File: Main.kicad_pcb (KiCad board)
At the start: 2 copper layers, 71.1 x 34.3 mm, 12 parts, among them P1 CONN_01X06, U3 BLE_NANO

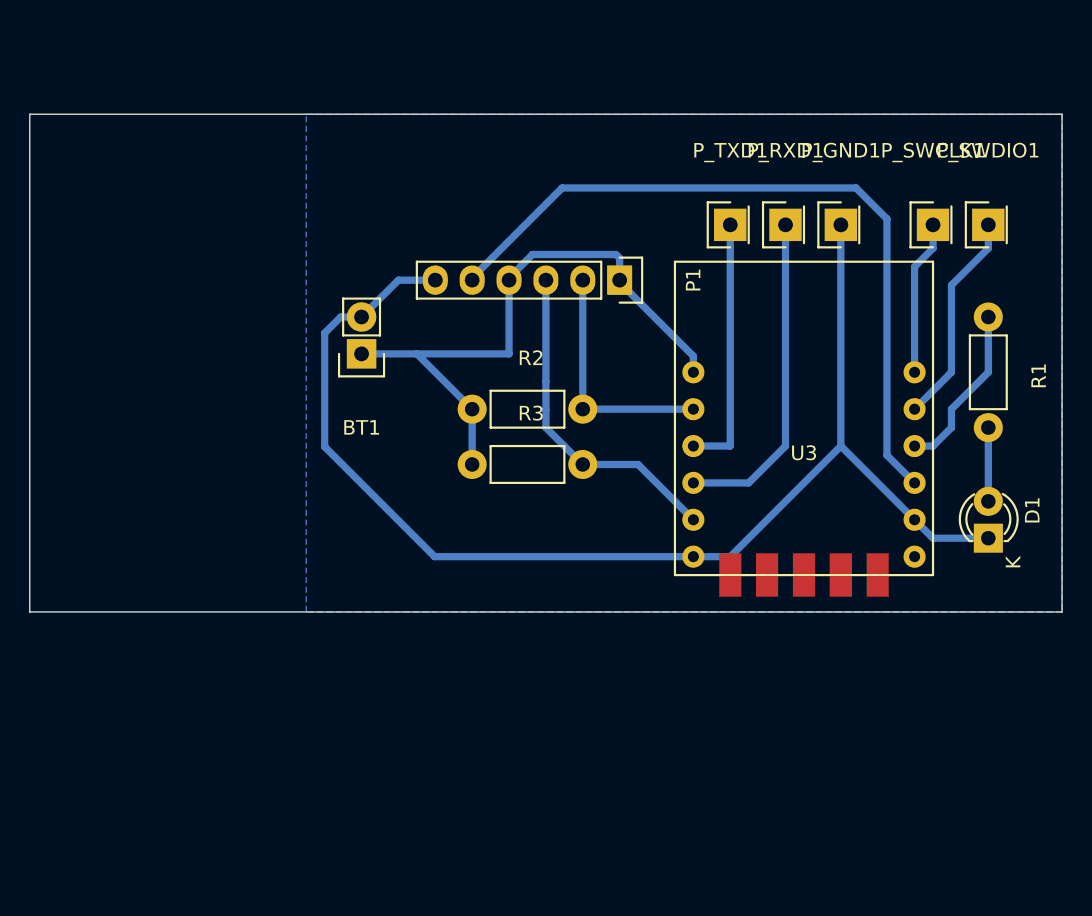
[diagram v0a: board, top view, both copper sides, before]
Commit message: update
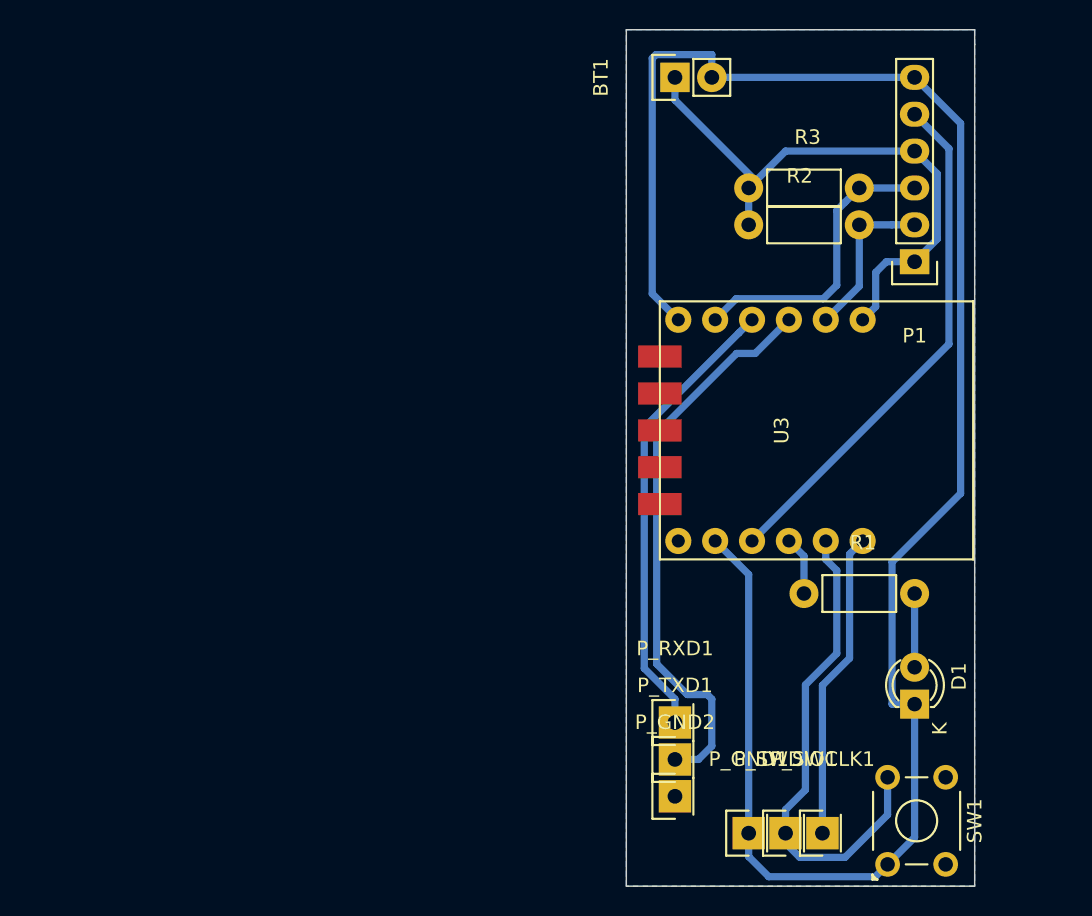
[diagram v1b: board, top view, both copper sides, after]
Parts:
- added P_GND2: CONN_01X01, Socket_Strips:Socket_Strip_Straight_1x01, F.Cu at (133.3, 130.8)
- added SW1: SW_RESET, Buttons_Switches_ThroughHole:SW_TH_Tactile_Omron_B3F-10xx, F.Cu at (148.0, 135.5)
- R1: value 10 -> 4.7k
- moved P_SWDIO1 44.2 mm to (141.0, 133.3)
- moved P_SWCLK1 42.6 mm to (143.5, 133.3)
- moved P_GND1 42.4 mm to (138.4, 133.3)
- moved P_TXD1 37.0 mm to (133.3, 128.3)
- moved P_RXD1 35.1 mm to (133.3, 125.7)
- moved BT1 28.8 mm to (133.3, 81.3), turned to 90 degrees
- moved R3 26.9 mm to (138.4, 88.9)
- moved R2 22.9 mm to (138.4, 91.4)
- moved R1 22.9 mm to (142.2, 116.8), turned to 0 degrees
- moved P1 20.4 mm to (149.9, 94.0), turned to 180 degrees
- moved D1 12.5 mm to (149.9, 124.5)
- moved U3 1.50 mm to (141.2, 105.6), turned to 270 degrees
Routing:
- net GND: track 86.8 -> 131.5 mm
- net /Main/TXD: track 17.8 -> 39.2 mm
- net /Main/SWDIO: track 14.8 -> 33.8 mm
- net INT: track 51.2 -> 36.0 mm
- net /Main/SWCLK: track 10.7 -> 21.3 mm
- net /Main/RXD: track 22.6 -> 31.7 mm
- net Net-(R1-Pad1): track 11.7 -> 4.05 mm
- net SDA: track 16.5 -> 11.3 mm
- net RESET: track 43.0 -> 40.0 mm
- net SCL: track 23.0 -> 20.5 mm
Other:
- board size 71.1 x 34.3 mm -> 24 x 59 mm
- net class Default: clearance 0.5 -> 0.3
- rule trace_clearance: 0.5 -> 0.3
